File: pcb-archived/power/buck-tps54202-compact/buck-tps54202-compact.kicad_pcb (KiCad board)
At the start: 2 copper layers, 37 x 18 mm, 32 parts, among them J1 Conn_01x03, J2 Conn_01x03, J3 Conn_01x03, J4 Conn_01x03, J5 Screw_Terminal_01x02, J6 Screw_Terminal_01x02, SW1 SW_DIP_x04, U1 TPS54202DDCR

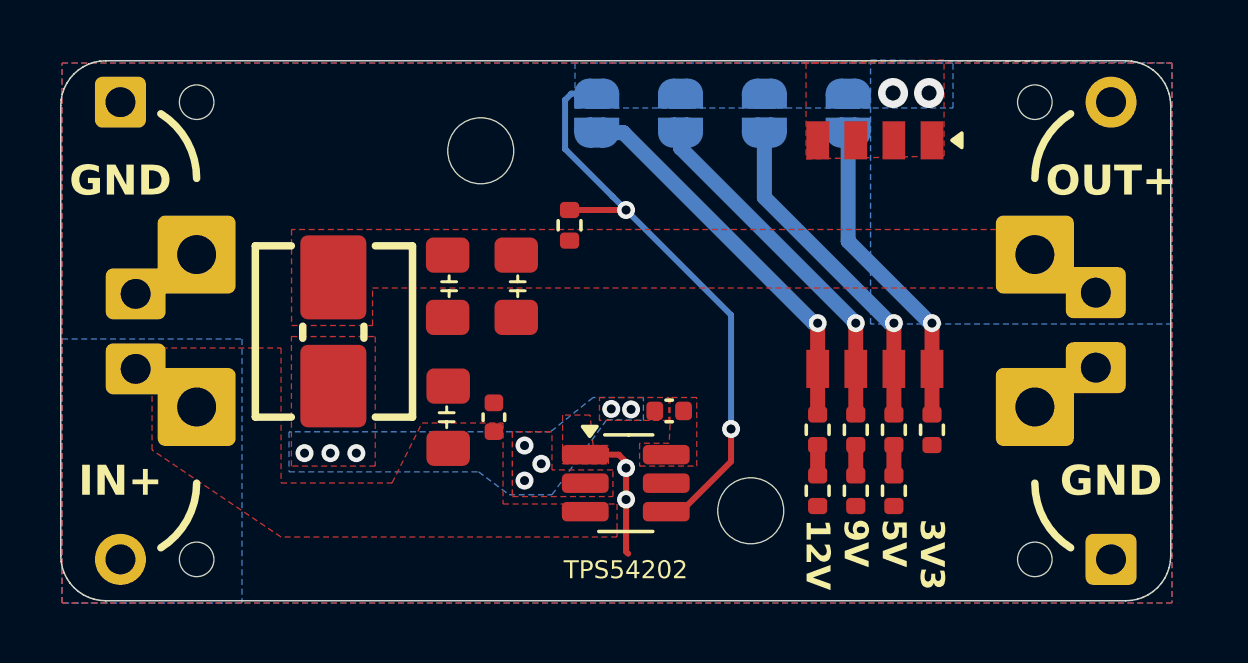
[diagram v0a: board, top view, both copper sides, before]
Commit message: Fix DRC warnings
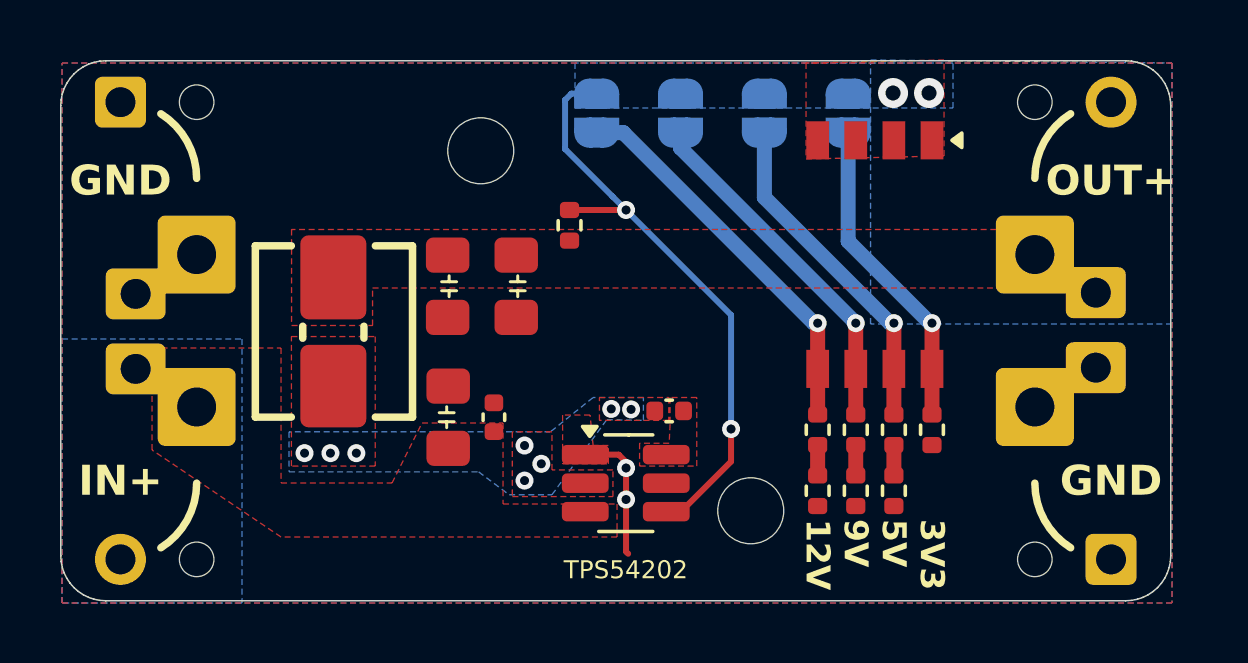
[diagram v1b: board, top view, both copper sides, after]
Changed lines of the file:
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@@
 			(size 2.2 2.75)
 			(layers "F.Cu" "F.Paste" "F.Mask")
-			(roundrect_rratio 0.1136363636)
+			(roundrect_rratio 0.125)
 			(net 5 "SW")
 			(pinfunction "1")
@@
 			(size 2.2 2.8)
 			(layers "F.Cu" "F.Paste" "F.Mask")
-			(roundrect_rratio 0.1136363636)
+			(roundrect_rratio 0.125)
 			(net 3 "VOUT")
 			(pinfunction "2")
